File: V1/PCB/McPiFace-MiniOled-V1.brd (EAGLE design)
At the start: 44 x 88 mm, 14 parts, among them J2 MC_PI_FACE_LEDSSIDE

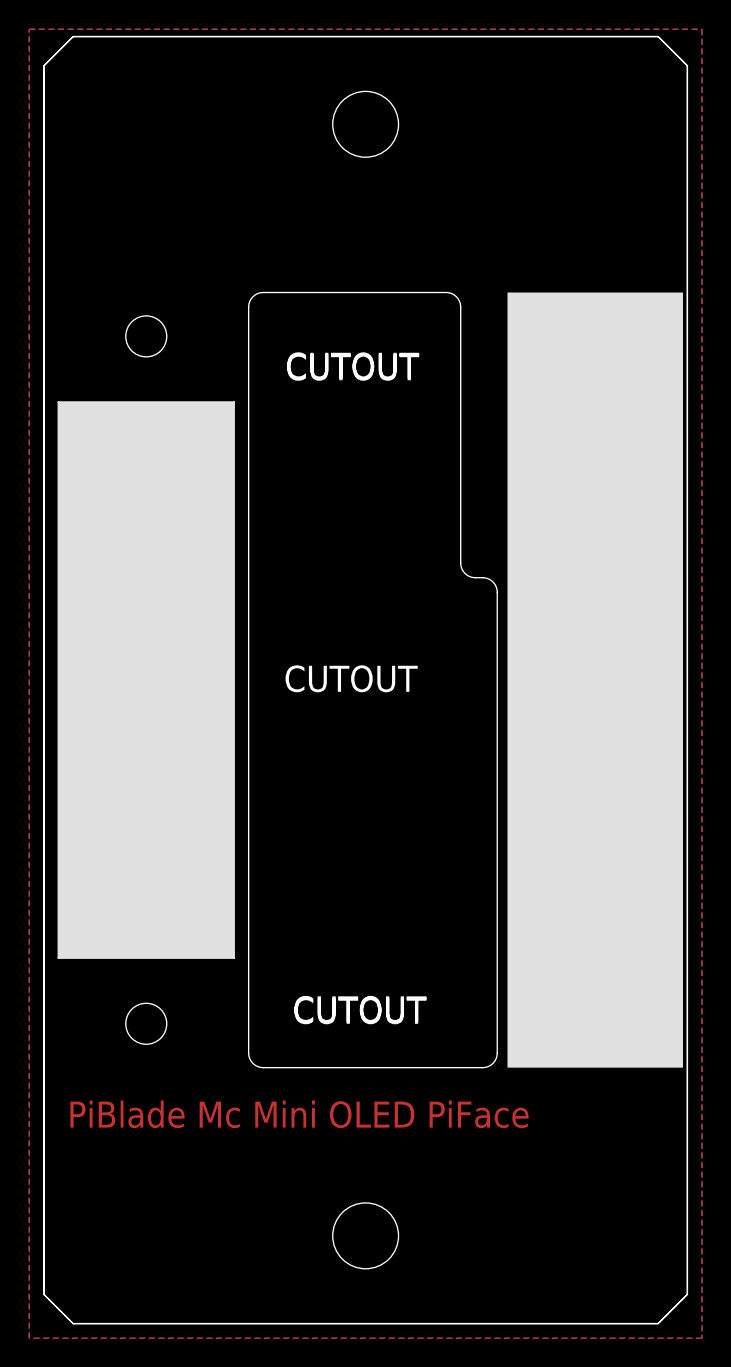
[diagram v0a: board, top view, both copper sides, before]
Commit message: Docs update.
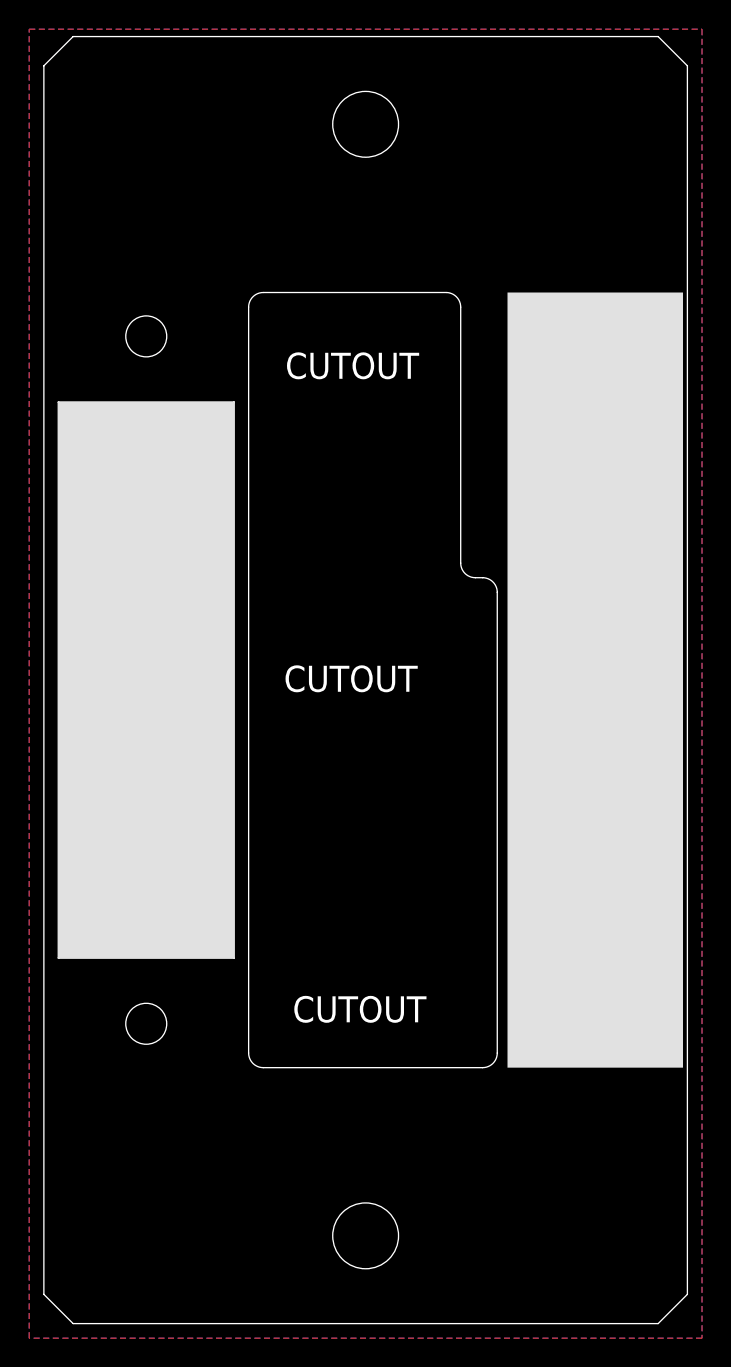
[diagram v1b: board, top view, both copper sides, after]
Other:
- outline, holes or cut-outs redrawn
- board text removed: "CUTOUT"
- board text removed: "PiBlade Mc Mini OLED PiFace"
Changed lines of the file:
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@@
 <board>
 <plain>
-<wire x1="2" y1="0" x2="42" y2="0" width="0" layer="20"/>
-<wire x1="42" y1="0" x2="44" y2="2" width="0" layer="20"/>
-<wire x1="44" y1="2" x2="44" y2="86" width="0" layer="20"/>
-<wire x1="44" y1="86" x2="42" y2="88" width="0" layer="20"/>
-<wire x1="42" y1="88" x2="2" y2="88" width="0" layer="20"/>
-<wire x1="2" y1="88" x2="0" y2="86" width="0" layer="20"/>
-<wire x1="0" y1="86" x2="0" y2="2" width="0" layer="20"/>
-<wire x1="0" y1="2" x2="2" y2="0" width="0" layer="20"/>
 <wire x1="22" y1="-6.5" x2="22" y2="108.5" width="0" layer="49"/>
 <wire x1="-3.5" y1="6" x2="51.5" y2="6" width="0" layer="49"/>
 <wire x1="-2" y1="82" x2="50" y2="82" width="0" layer="49"/>
-<text x="16.5" y="64.5" size="1.778" layer="20">CUTOUT</text>
-<text x="17" y="20.5" size="1.778" layer="20">CUTOUT</text>
 <dimension x1="14" y1="17.5" x2="14" y2="0" x3="14" y3="8.75" textsize="1.778" layer="47"/>
 <dimension x1="14" y1="17.5" x2="0" y2="17.5" x3="7" y3="-8.5" textsize="1.778" layer="47"/>
@@
 <wire x1="-1.5" y1="76" x2="50" y2="76" width="0.4064" layer="49"/>
 <wire x1="-3.5" y1="12" x2="51.5" y2="12" width="0.4064" layer="49"/>
-<text x="1.6" y="13.4" size="1.778" layer="1" ratio="15">PiBlade Mc Mini OLED PiFace</text>
 <text x="33.6" y="58.8" size="1.27" layer="26" ratio="15" rot="MR270">https://github.com/McPiFace/MiniOled</text>
 <circle x="22" y="82" radius="5" width="0.2" layer="41"/>
@@
 </class>
 </classes>
-<designrules name="dirt_cheap_dirty_boards.v1">
+<designrules name="dirt_cheap_dirty_boards.v1.1">
+<description language="de">&lt;b&gt;Dirty Cheap Dirty Board Design Rules&lt;/b&gt;
+&lt;br&gt;
+&lt;br&gt;Min width/Spacing: 6/6mil
+&lt;br&gt;Min diameter of finished hole 12mil</description>
 <description language="en">&lt;b&gt;Dirty Cheap Dirty Board Design Rules&lt;/b&gt;
 &lt;br&gt;
-&lt;br&gt;Min width/Spacing: 5/5mil
+&lt;br&gt;Min width/Spacing: 6/6mil
+&lt;br&gt;Min diameter of finished hole 12mil</description>
+<description language="zh">&lt;b&gt;Dirty Cheap Dirty Board Design Rules&lt;/b&gt;
+&lt;br&gt;
+&lt;br&gt;Min width/Spacing: 6/6mil
 &lt;br&gt;Min diameter of finished hole 12mil</description>
 <param name="layerSetup" value="(1*16)"/>
 <param name="mtCopper" value="0.035mm 0.0175mm 0.035mm 0.035mm 0.035mm 0.035mm 0.035mm 0.035mm 0.035mm 0.035mm 0.035mm 0.035mm 0.035mm 0.035mm 0.0175mm 0.035mm"/>
 <param name="mtIsolate" value="1.5mm 1.1mm 0.2mm 0.15mm 0.2mm 0.15mm 0.2mm 0.15mm 0.2mm 0.15mm 0.2mm 0.15mm 0.2mm 0.15mm 0.2mm"/>
-<param name="mdWireWire" value="5mil"/>
-<param name="mdWirePad" value="5mil"/>
-<param name="mdWireVia" value="5mil"/>
-<param name="mdPadPad" value="5mil"/>
-<param name="mdPadVia" value="5mil"/>
-<param name="mdViaVia" value="5mil"/>
+<param name="mdWireWire" value="6mil"/>
+<param name="mdWirePad" value="6mil"/>
+<param name="mdWireVia" value="6mil"/>
+<param name="mdPadPad" value="6mil"/>
+<param name="mdPadVia" value="6mil"/>
+<param name="mdViaVia" value="6mil"/>
 <param name="mdSmdPad" value="0mil"/>
 <param name="mdSmdVia" value="0mil"/>
@@
 <param name="mdDrill" value="10mil"/>
 <param name="mdSmdStop" value="0mil"/>
-<param name="msWidth" value="5mil"/>
+<param name="msWidth" value="6mil"/>
 <param name="msDrill" value="12mil"/>
 <param name="msMicroVia" value="12mil"/>
